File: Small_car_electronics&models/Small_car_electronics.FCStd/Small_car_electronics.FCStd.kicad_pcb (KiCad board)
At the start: 2 copper layers, 58.5 x 74.5 mm, 10 parts

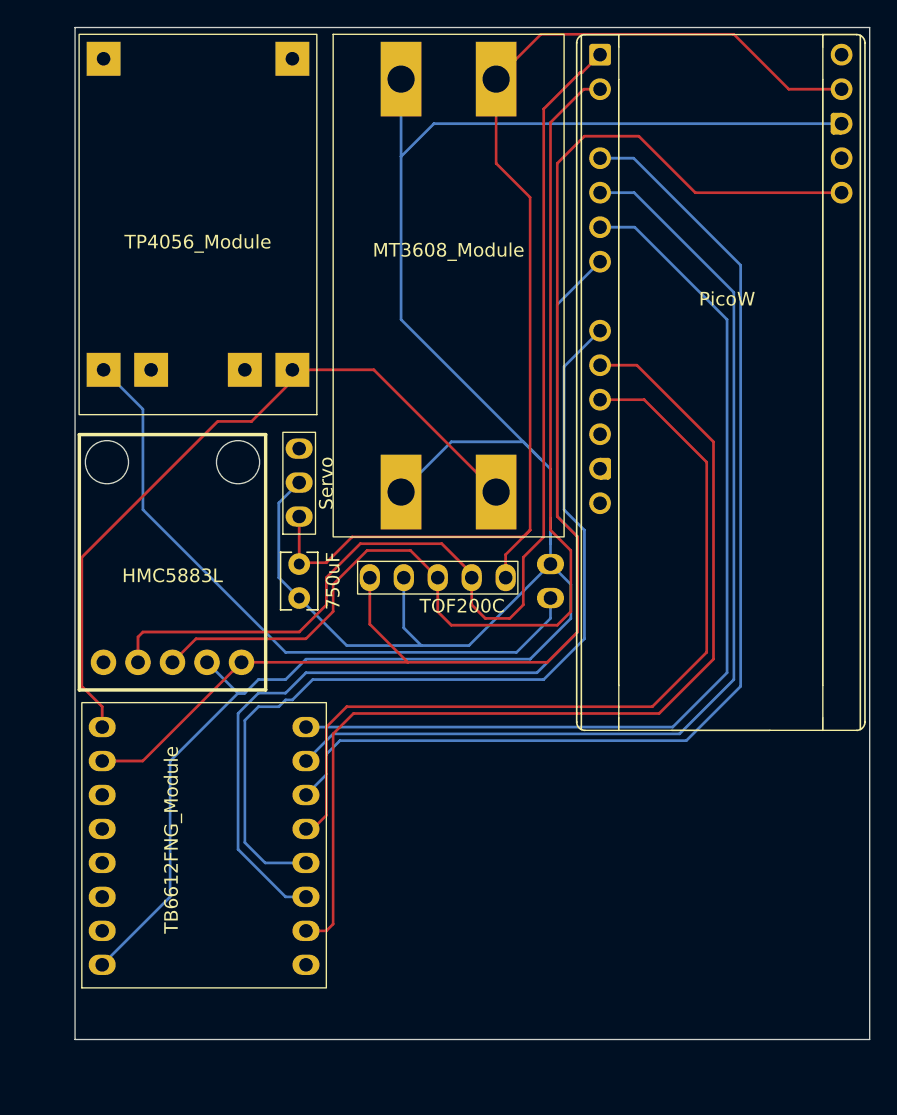
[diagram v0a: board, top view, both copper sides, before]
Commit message: Updated design
Created better design for car shell and
car PCB, removed compass and changed plastic tracks to rubber belt.
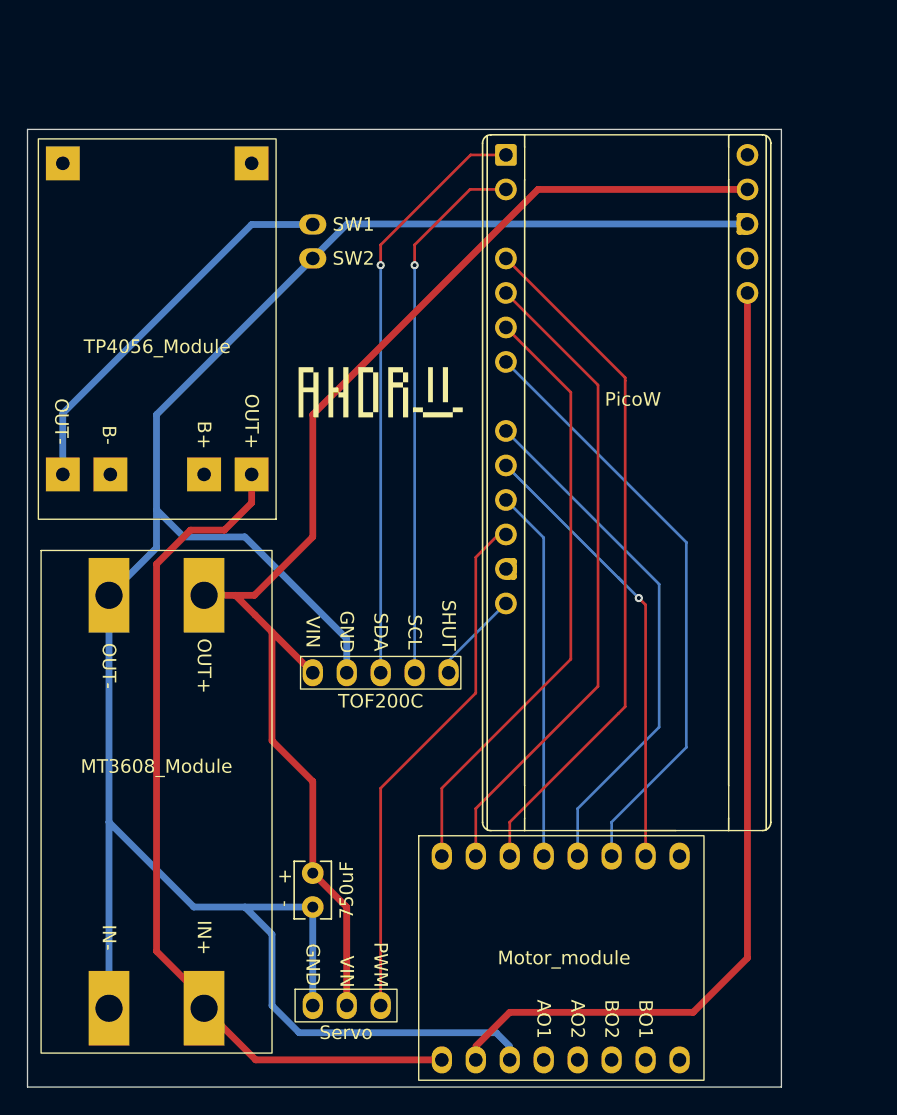
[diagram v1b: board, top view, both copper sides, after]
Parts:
- removed HMC5883L: HMC5883L, CustomFutprints:HMC5883L
- added G***: LOGO, logo:mylogo, F.Cu at (93.5, 66.5)
- moved MT3608_Module 43.7 mm to (78.5, 88.0)
- moved Servo 41.2 mm to (91.0, 114.2), turned to 0 degrees
- moved ? 30.5 mm to (88.5, 56.5)
- moved ? 30.5 mm to (88.5, 54.0)
- moved TB6612FNG_Module 30.1 mm to (107.8, 106.2), turned to 0 degrees
- moved 750uF 22.8 mm to (88.5, 104.2)
- moved PicoW 10.1 mm to (112.1, 67.4)
- moved TP4056_Module 8.26 mm to (77.8, 61.7)
- moved TOF200C 8.16 mm to (95.3, 90.6)
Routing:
- net (no net): track 1143.8 -> 848.4 mm, vias 0 -> 3
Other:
- board size 58.5 x 74.5 mm -> 55.5 x 70.5 mm
- board text added: "+"
- board text added: "-"
- board text added: "AO1"
- board text added: "AO2"
- board text added: "B+"
- board text added: "B-"
- board text added: "BO1"
- board text added: "BO2"
- board text added: "GND"
- board text added: "IN+"
- board text added: "IN-"
- board text added: "Motor_module"
- board text added: "OUT+"
- board text added: "OUT-"
- board text added: "PWM"
- board text added: "SCL"
- board text added: "SDA"
- board text added: "SHUT"
- board text added: "SW1"
- board text added: "SW2"
- board text added: "VIN"
